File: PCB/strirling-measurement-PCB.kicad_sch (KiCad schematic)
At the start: 7 parts, among them J1 NTC_Connector1, J2 NTC_Connector2, J3 NTC_Connector3, J4 NTC_Connector4, J5 NTC_Connector1, U1 NUCLEO-G431KB

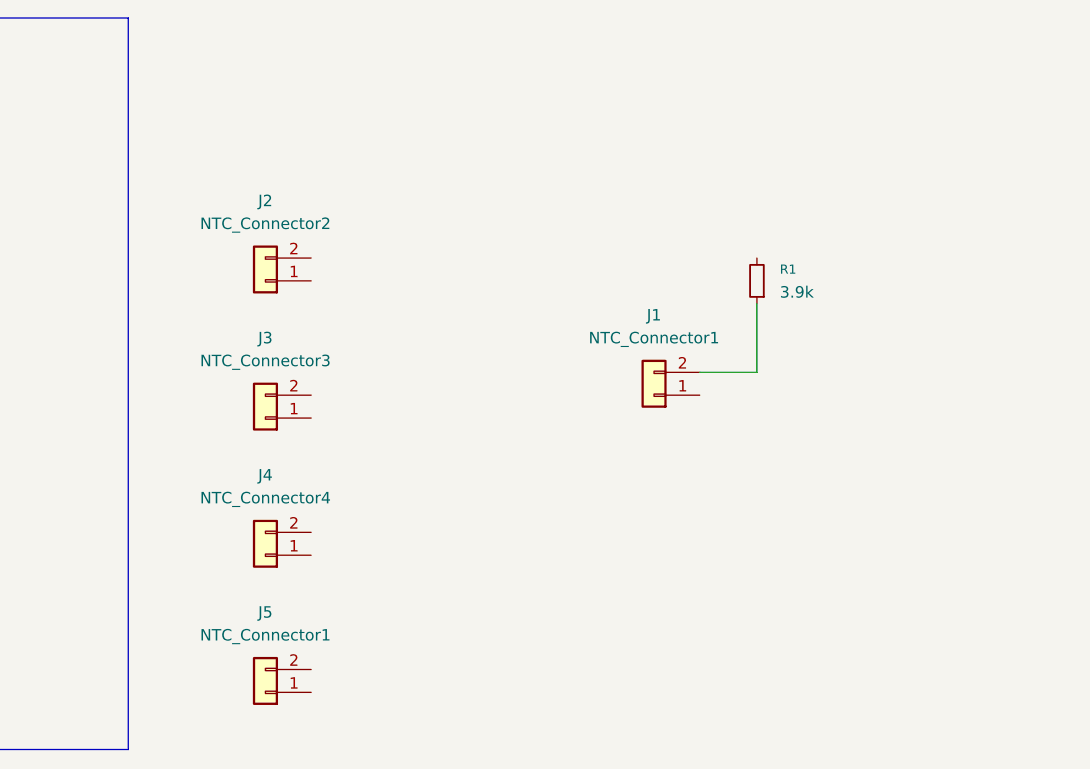
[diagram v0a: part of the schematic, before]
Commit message: -
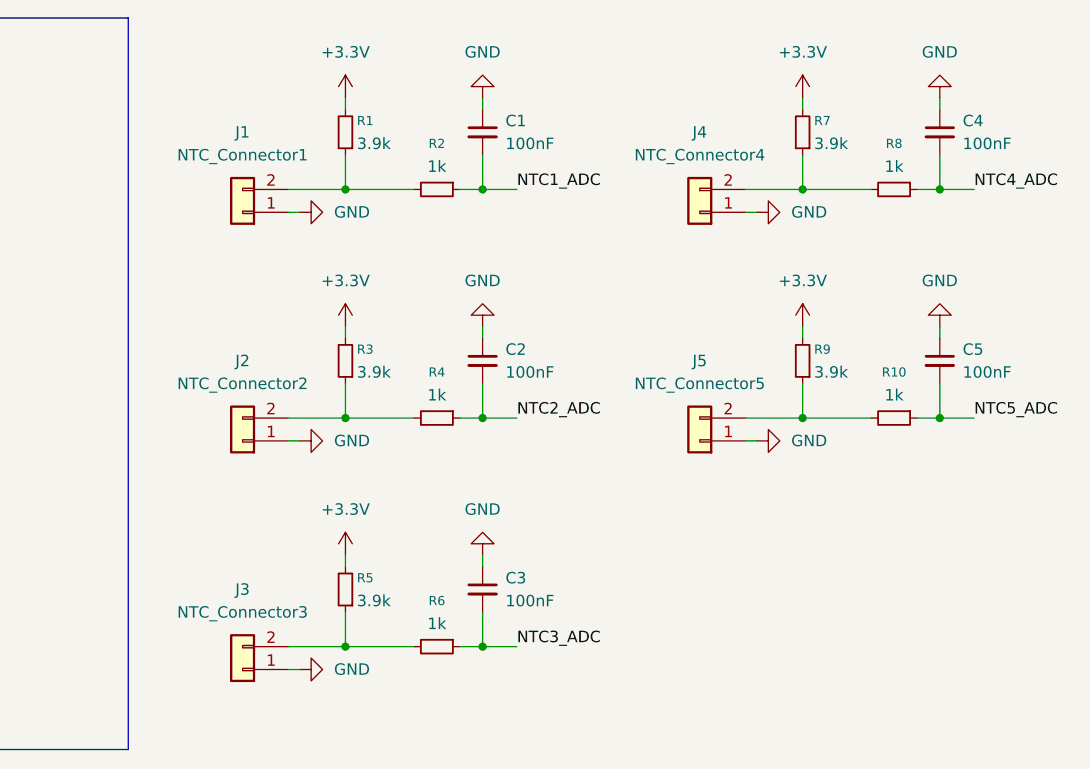
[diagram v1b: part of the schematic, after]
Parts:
- added C1, C2, C3, C4, C5: 100nF, symbol Device:C_Small
- added R10, R2, R4, R6, R8: 1k, symbol Device:R_Small
- added R3, R5, R7, R9: 3.9k, symbol Device:R_Small
- J5: value NTC_Connector1 -> NTC_Connector5
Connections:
- net GND: now reaches J4.1 (Pin_1)
- net GND: now also J1.1 (Pin_1), J2.1 (Pin_1), J3.1 (Pin_1), J5.1 (Pin_1), C1.1, C2.1, C3.1, C4.1, C5.1
- net at J4.2 (Pin_2): now also R7.1, R8.2
- net at J5.2 (Pin_2): now also R10.2, R9.1
- net at J1.2 (Pin_2), R1.1: now also R2.2
- net +3.3V: now reaches R1.2
- net +3.3V: now also R3.2, R5.2, R7.2, R9.2
- net at J2.2 (Pin_2): now also R3.1, R4.2
- net at J3.2 (Pin_2): now also R5.1, R6.2
- new net NTC1_ADC: C1.2, R2.1
- new net NTC2_ADC: C2.2, R4.1
- new net NTC3_ADC: C3.2, R6.1
- new net NTC4_ADC: C4.2, R8.1
- new net NTC5_ADC: C5.2, R10.1
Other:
- moved on the sheet: J1, J2, J3, J4, J5, R1

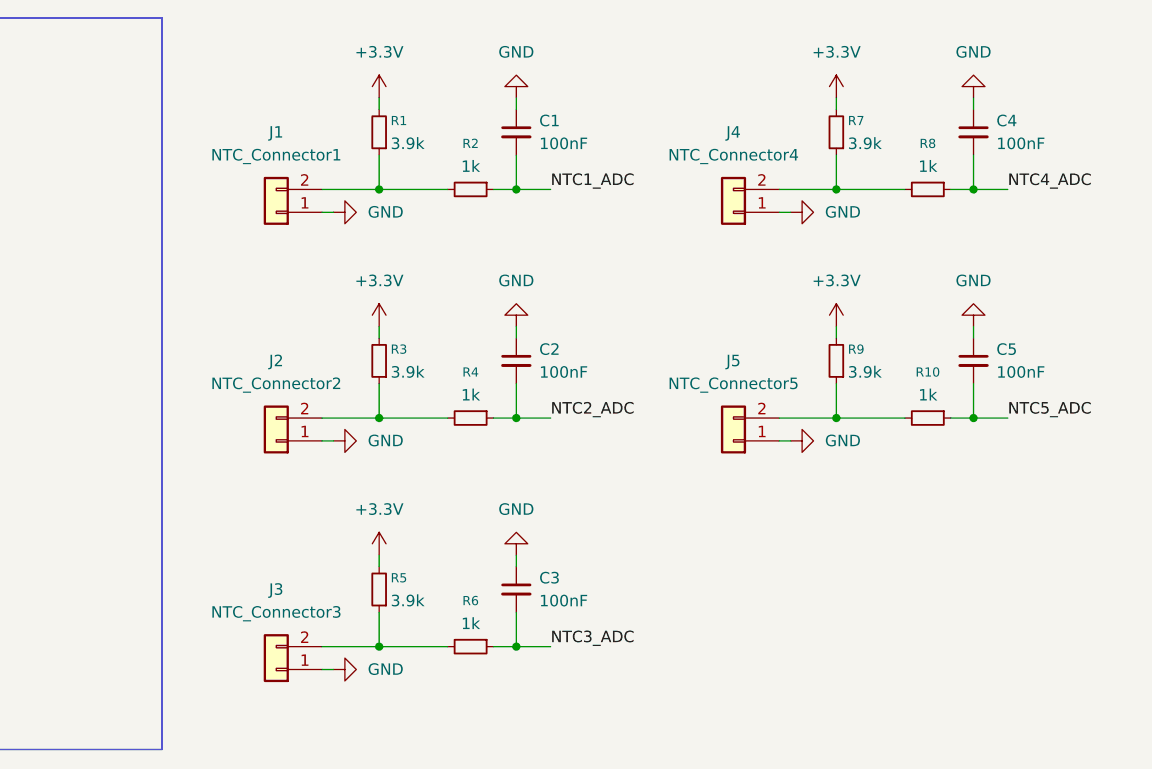
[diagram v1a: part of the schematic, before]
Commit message: -
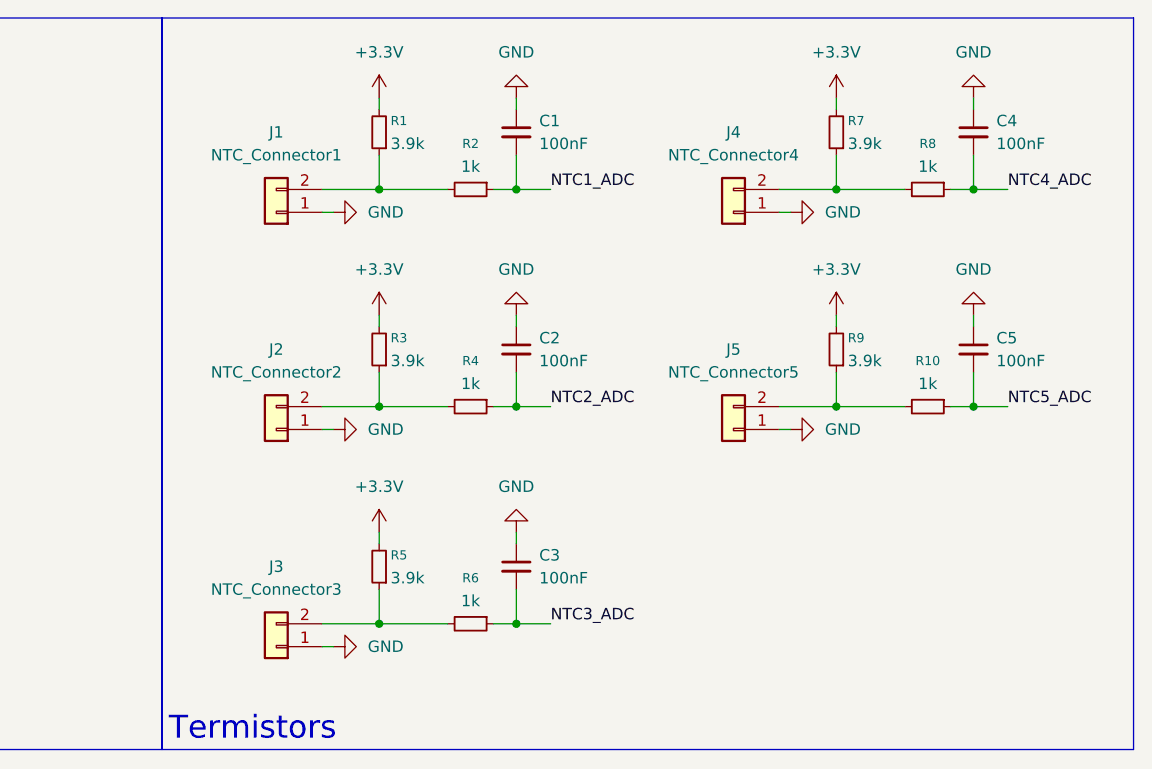
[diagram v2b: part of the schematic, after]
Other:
- note added: "Termistors"
- moved on the sheet: C2, C3, C5, J2, J3, J5, R10, R3, R4, R5, R6, R9

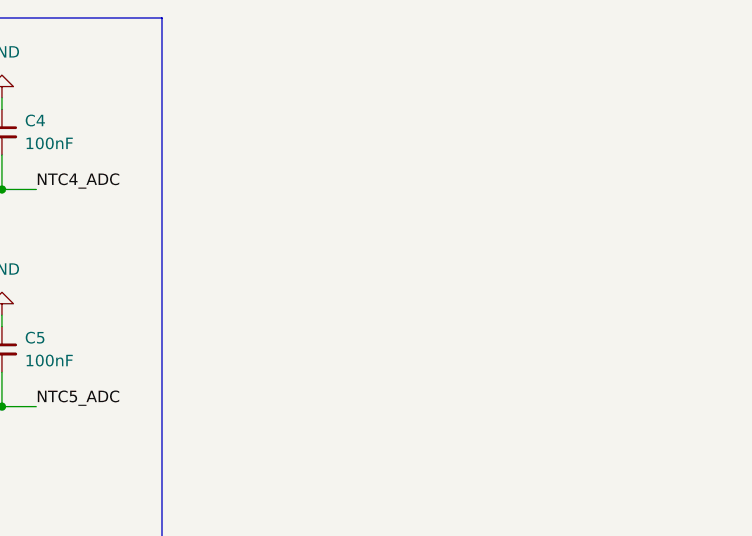
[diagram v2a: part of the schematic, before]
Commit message: -
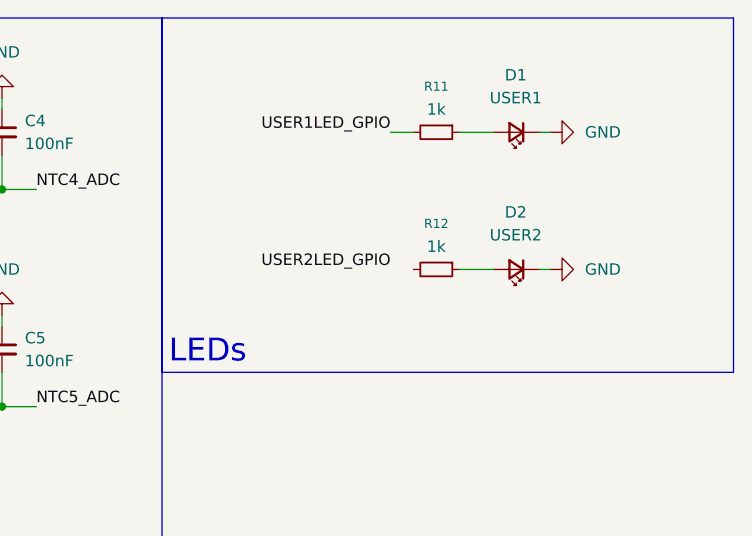
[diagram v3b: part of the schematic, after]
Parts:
- added D1: USER1, LED_THT:LED_D5.0mm_FlatTop, symbol Device:LED_Small
- added D2: USER2, LED_THT:LED_D5.0mm_FlatTop, symbol Device:LED_Small
- added R11, R12: 1k, Resistor_SMD:R_0805_2012Metric, symbol Device:R_Small
- C1, C2, C3, C4, C5: footprint (none) -> Capacitor_SMD:C_0805_2012Metric
- J1, J2, J3, J4, J5: footprint (none) -> stirling-measurement-PCB-footprintlibrary:JST_S2B-ZR_LF__SN_
- R1, R3, R5, R7, R9: footprint (none) -> Resistor_SMD:R_0603_1608Metric
- R10, R2, R4, R6, R8: footprint (none) -> Resistor_SMD:R_0805_2012Metric
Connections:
- net GND: now also D1.1 (K), D2.1 (K)
- new net: D1.2 (A), R11.1
- new net: D2.2 (A), R12.1
- new net USER1LED_GPIO: R11.2
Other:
- note added: "LEDs"

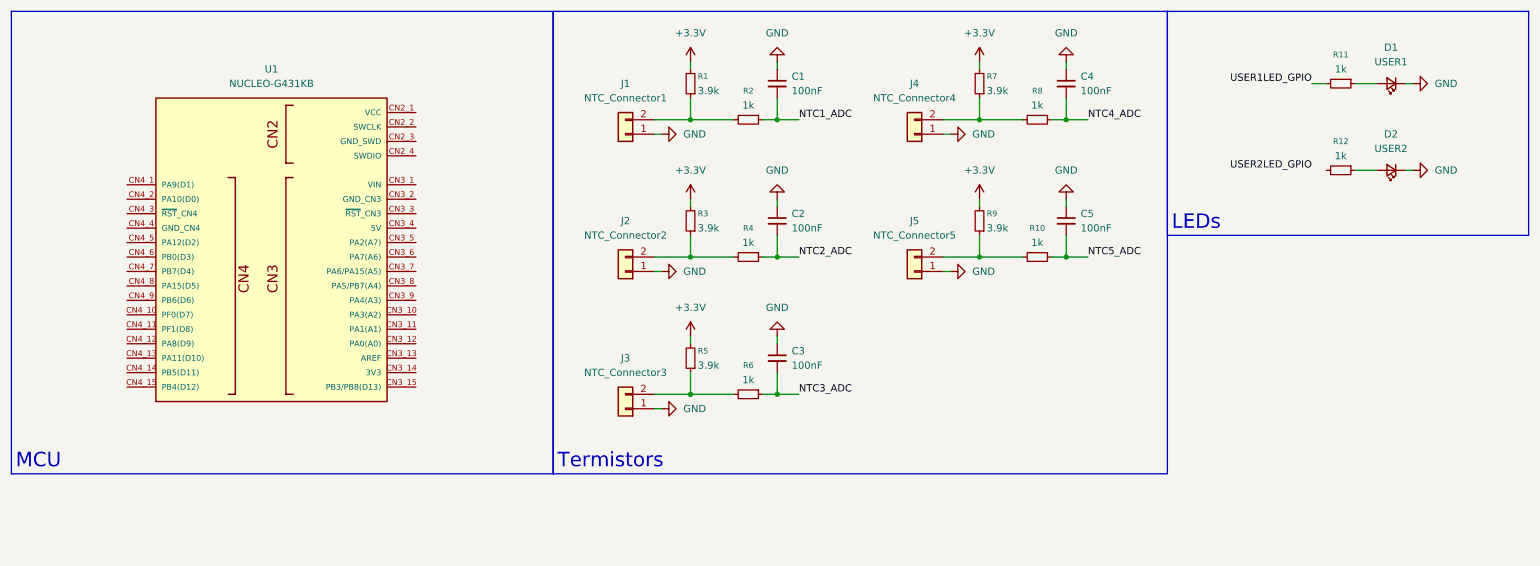
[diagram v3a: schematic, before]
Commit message: ready
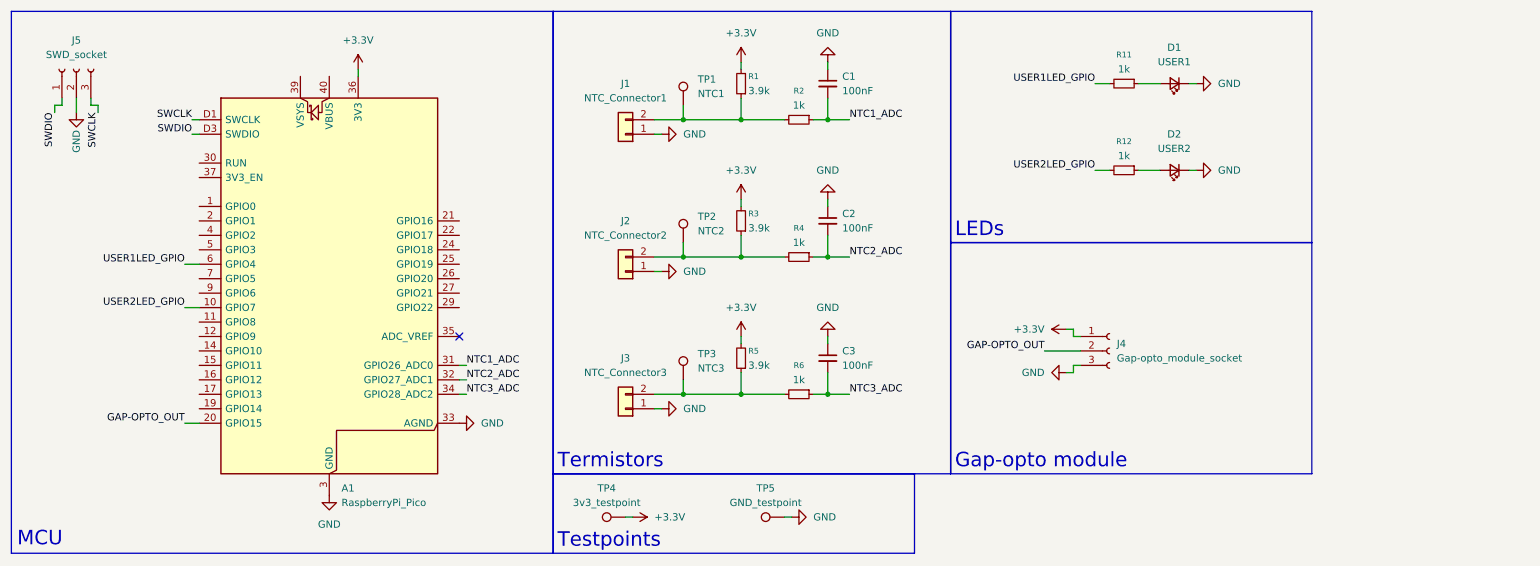
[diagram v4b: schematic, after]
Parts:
- removed C4, C5: 100nF, Capacitor_SMD:C_0805_2012Metric, symbol Device:C_Small
- removed J4: NTC_Connector4, stirling-measurement-PCB-footprintlibrary:JST_S2B-ZR_LF__SN_, symbol Connector_Generic:Conn_01x02
- removed J5: NTC_Connector5, stirling-measurement-PCB-footprintlibrary:JST_S2B-ZR_LF__SN_, symbol Connector_Generic:Conn_01x02
- removed R10, R8: 1k, Resistor_SMD:R_0805_2012Metric, symbol Device:R_Small
- removed R7, R9: 3.9k, Resistor_SMD:R_0603_1608Metric, symbol Device:R_Small
- removed U1: NUCLEO-G431KB, stirling-measurement-PCB-footprintlibrary:MODULE_NUCLEO-G431KB, symbol stirlling-measurement-PCB-symbollibrary:NUCLEO-G431KB
- added A1: RaspberryPi_Pico, Module:RaspberryPi_Pico_SMD_HandSolder, symbol MCU_Module:RaspberryPi_Pico_Debug
- added J4: Gap-opto_module_socket, stirling-measurement-PCB-footprintlibrary:gap-opto_module, symbol Connector:Conn_01x03_Socket
- added J5: SWD_socket, stirling-measurement-PCB-footprintlibrary:swd_header, symbol Connector:Conn_01x03_Socket
- added TP1: NTC1, TestPoint:TestPoint_Pad_2.0x2.0mm, symbol Connector:TestPoint
- added TP2: NTC2, TestPoint:TestPoint_Pad_2.0x2.0mm, symbol Connector:TestPoint
- added TP3: NTC3, TestPoint:TestPoint_Pad_2.0x2.0mm, symbol Connector:TestPoint
- added TP4: 3v3_testpoint, TestPoint:TestPoint_Pad_2.0x2.0mm, symbol Connector:TestPoint
- added TP5: GND_testpoint, TestPoint:TestPoint_Pad_2.0x2.0mm, symbol Connector:TestPoint
- C1, C2, C3: footprint Capacitor_SMD:C_0805_2012Metric -> Capacitor_SMD:C_0402_1005Metric
- D1, D2: footprint LED_THT:LED_D5.0mm_FlatTop -> LED_THT:LED_D5.0mm
- R2, R4, R6: footprint Resistor_SMD:R_0805_2012Metric -> Resistor_SMD:R_0402_1005Metric
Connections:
- net +3.3V: now also A1.36 (3V3), J4.1 (Pin_1), TP4.1
- net GND: now also A1.13 (GND), A1.18 (GND), A1.23 (GND), A1.28 (GND), A1.3 (GND), A1.33 (AGND), A1.38 (GND), A1.8 (GND), A1.D2 (GND), J4.3 (Pin_3), J5.2 (Pin_2), TP5.1
- net NTC1_ADC: now also A1.31 (GPIO26_ADC0)
- net NTC2_ADC: now also A1.32 (GPIO27_ADC1)
- net NTC3_ADC: now also A1.34 (GPIO28_ADC2)
- net USER1LED_GPIO: now also A1.6 (GPIO4)
- net USER2LED_GPIO: now also R12.2, A1.10 (GPIO7)
- net at J3.2 (Pin_2), R5.1, R6.2: now also TP3.1
- net at J1.2 (Pin_2), R1.1, R2.2: now also TP1.1
- net at J2.2 (Pin_2), R3.1, R4.2: now also TP2.1
- new net GAP-OPTO_OUT: A1.20 (GPIO15), J4.2 (Pin_2)
- new net SWCLK: A1.D1 (SWCLK), J5.3 (Pin_3)
- new net SWDIO: A1.D3 (SWDIO), J5.1 (Pin_1)
- no-connect marks 0 -> 1
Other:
- note added: "Gap-opto module"
- note added: "Testpoints"
- company: Berzsenyi Dániel GImnázium -> Berzsenyi Dániel Gimnázium
- moved on the sheet: C1, C2, C3, D1, D2, R1, R11, R12, R2, R3, R4, R5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
